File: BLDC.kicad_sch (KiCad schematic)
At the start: 1 part, among them U3 MIC4604YM

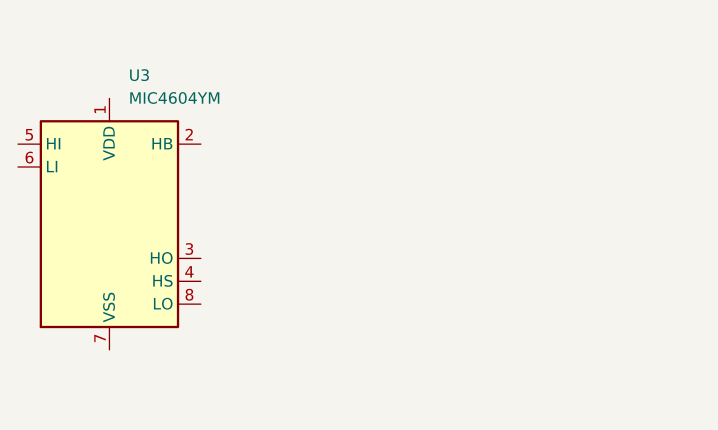
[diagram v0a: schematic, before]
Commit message: Can aangesloten
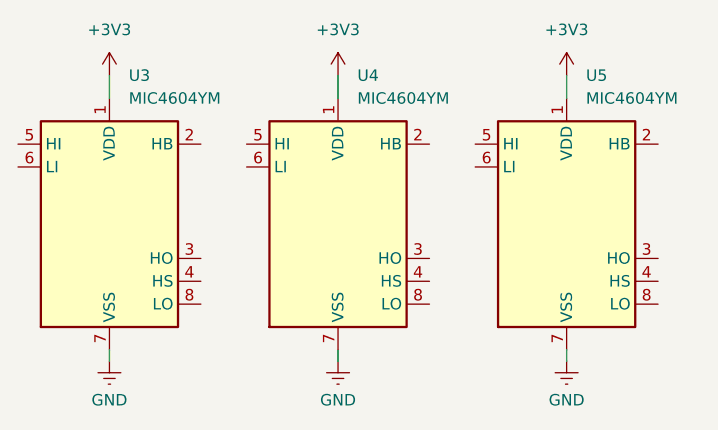
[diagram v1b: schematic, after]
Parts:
- added U4, U5: MIC4604YM, Package_SO:SOIC-8_3.9x4.9mm_P1.27mm, symbol Driver_FET:MIC4604YM
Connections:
- net +3V3: now reaches U3.1 (VDD)
- net +3V3: now also U4.1 (VDD), U5.1 (VDD)
- net GND: now reaches U3.7 (VSS)
- net GND: now also U4.7 (VSS), U5.7 (VSS)
